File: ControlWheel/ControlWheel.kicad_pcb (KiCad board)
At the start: 2 copper layers, 80.5 x 52 mm, 14 parts, among them J1 Conn_01x06_Pin, U1 AI12

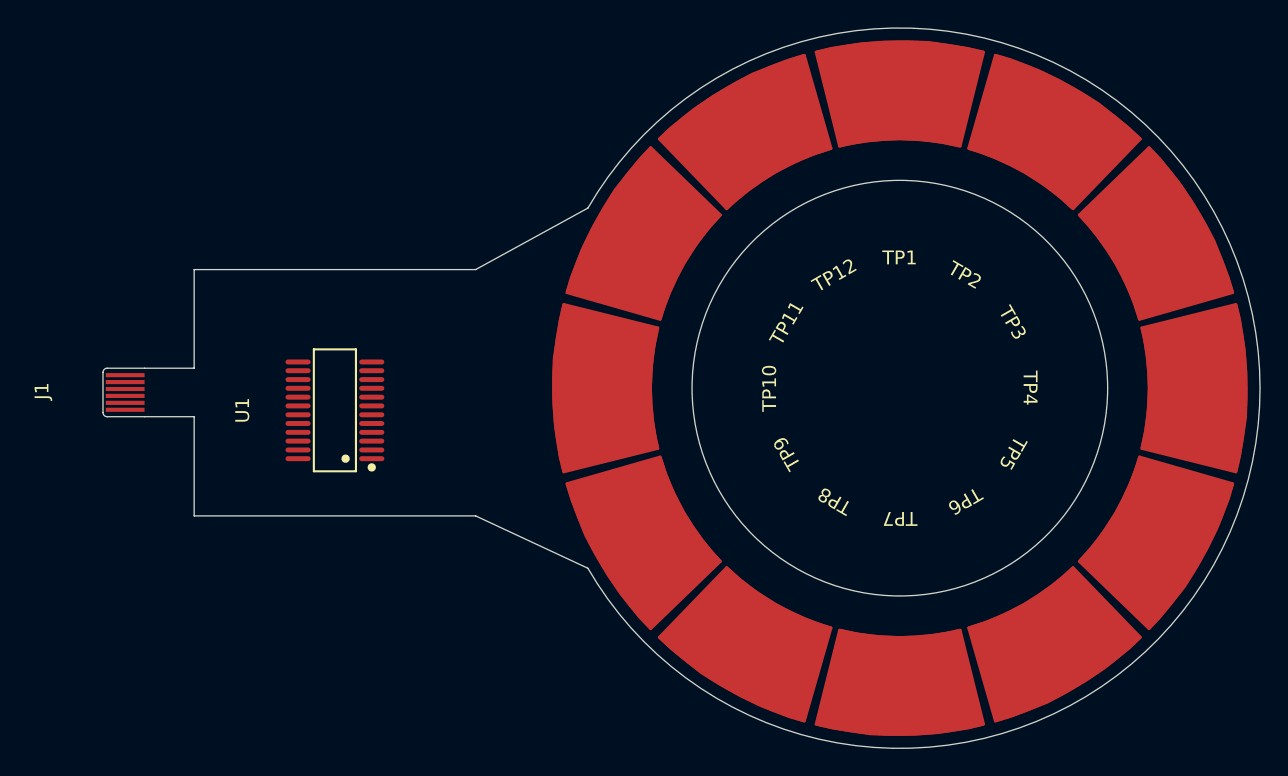
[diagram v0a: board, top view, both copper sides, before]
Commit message: minor power changes
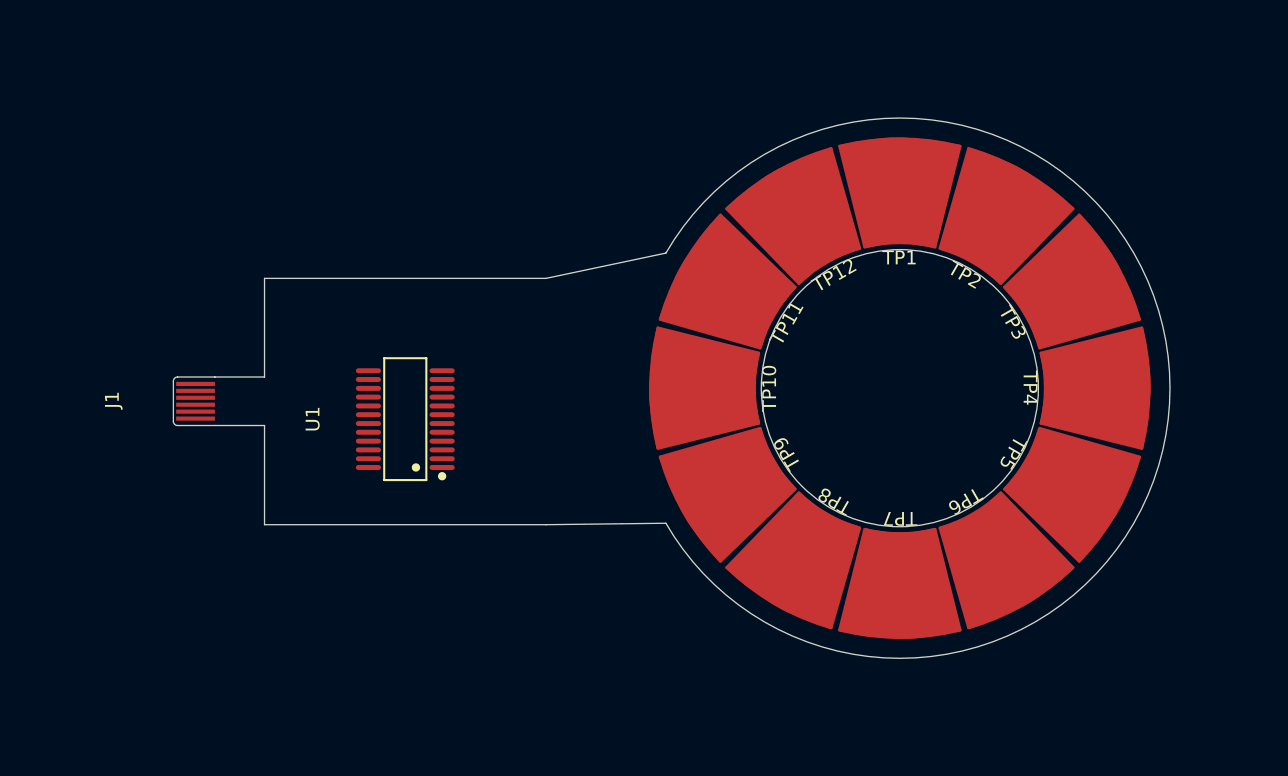
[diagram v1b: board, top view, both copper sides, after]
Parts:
- moved U1 5.12 mm to (114.3, 102.2)
- moved J1 5.12 mm to (97.6, 100.9)
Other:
- board size 80.5 x 52 mm -> 68.9 x 39 mm
